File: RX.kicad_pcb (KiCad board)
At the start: 2 copper layers, 131.3 x 71.3 mm, 27 parts, among them J1 Conn_01x03, J2 Screw_Terminal_01x06, J3 Conn_01x03, J4 Conn_01x04, J5 Conn_01x04, J6 Conn_01x04, Q1 BC547, Q2 BC547, U1 ESP32-DEVKIT-V1

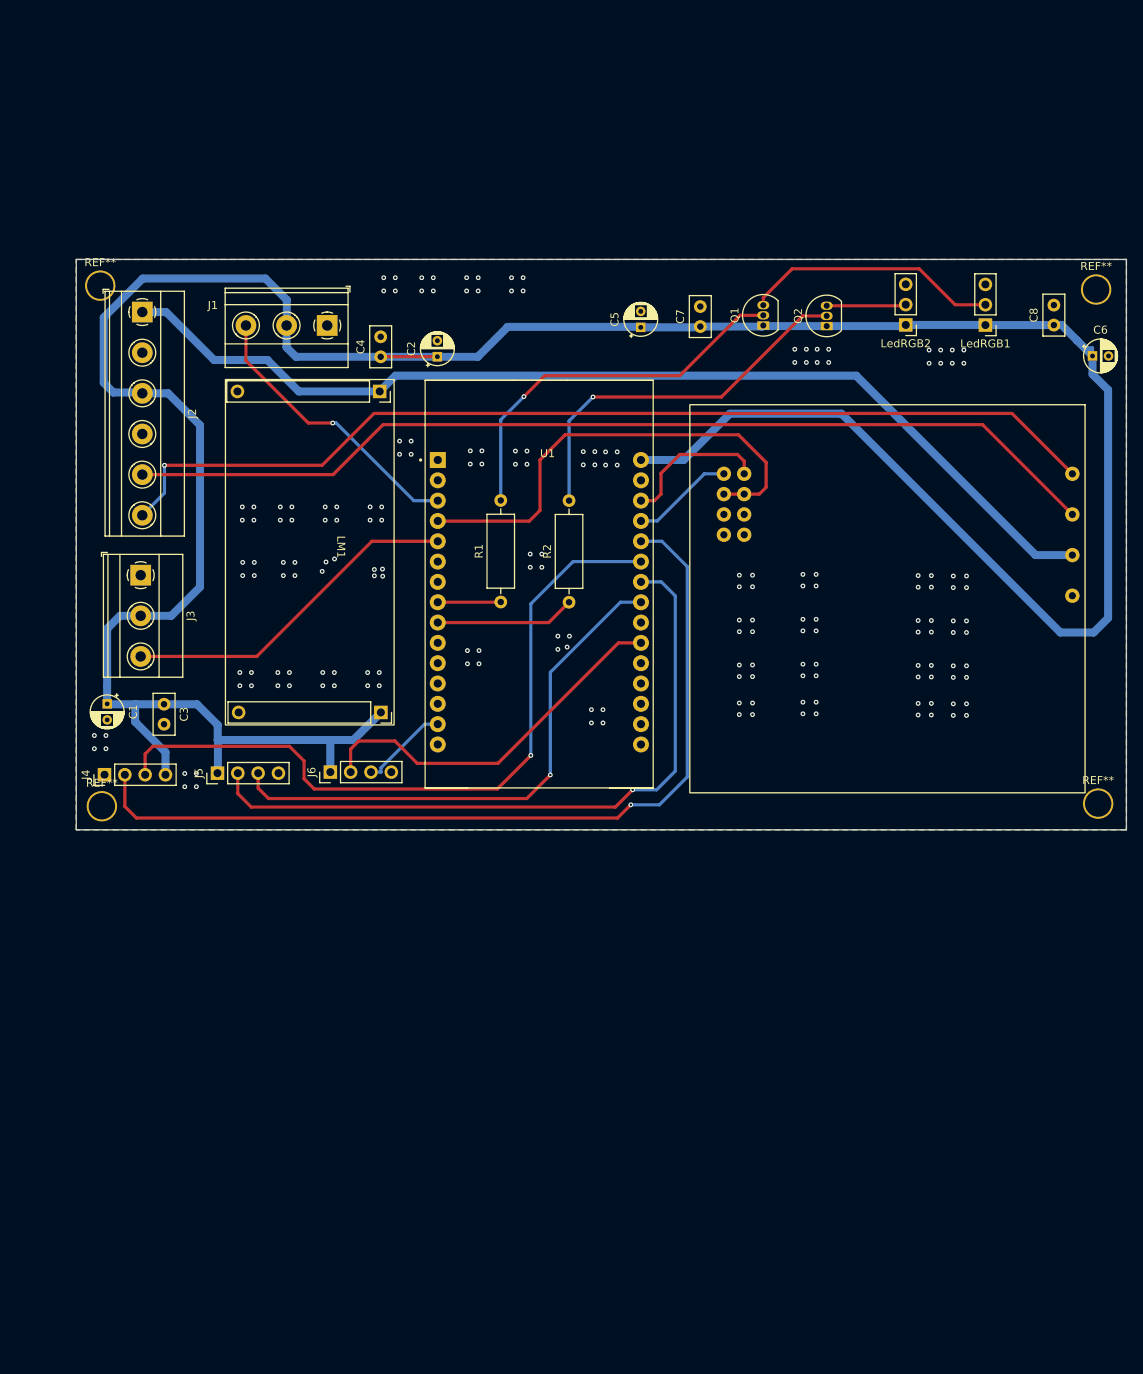
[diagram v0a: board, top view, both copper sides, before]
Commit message: Add files via upload
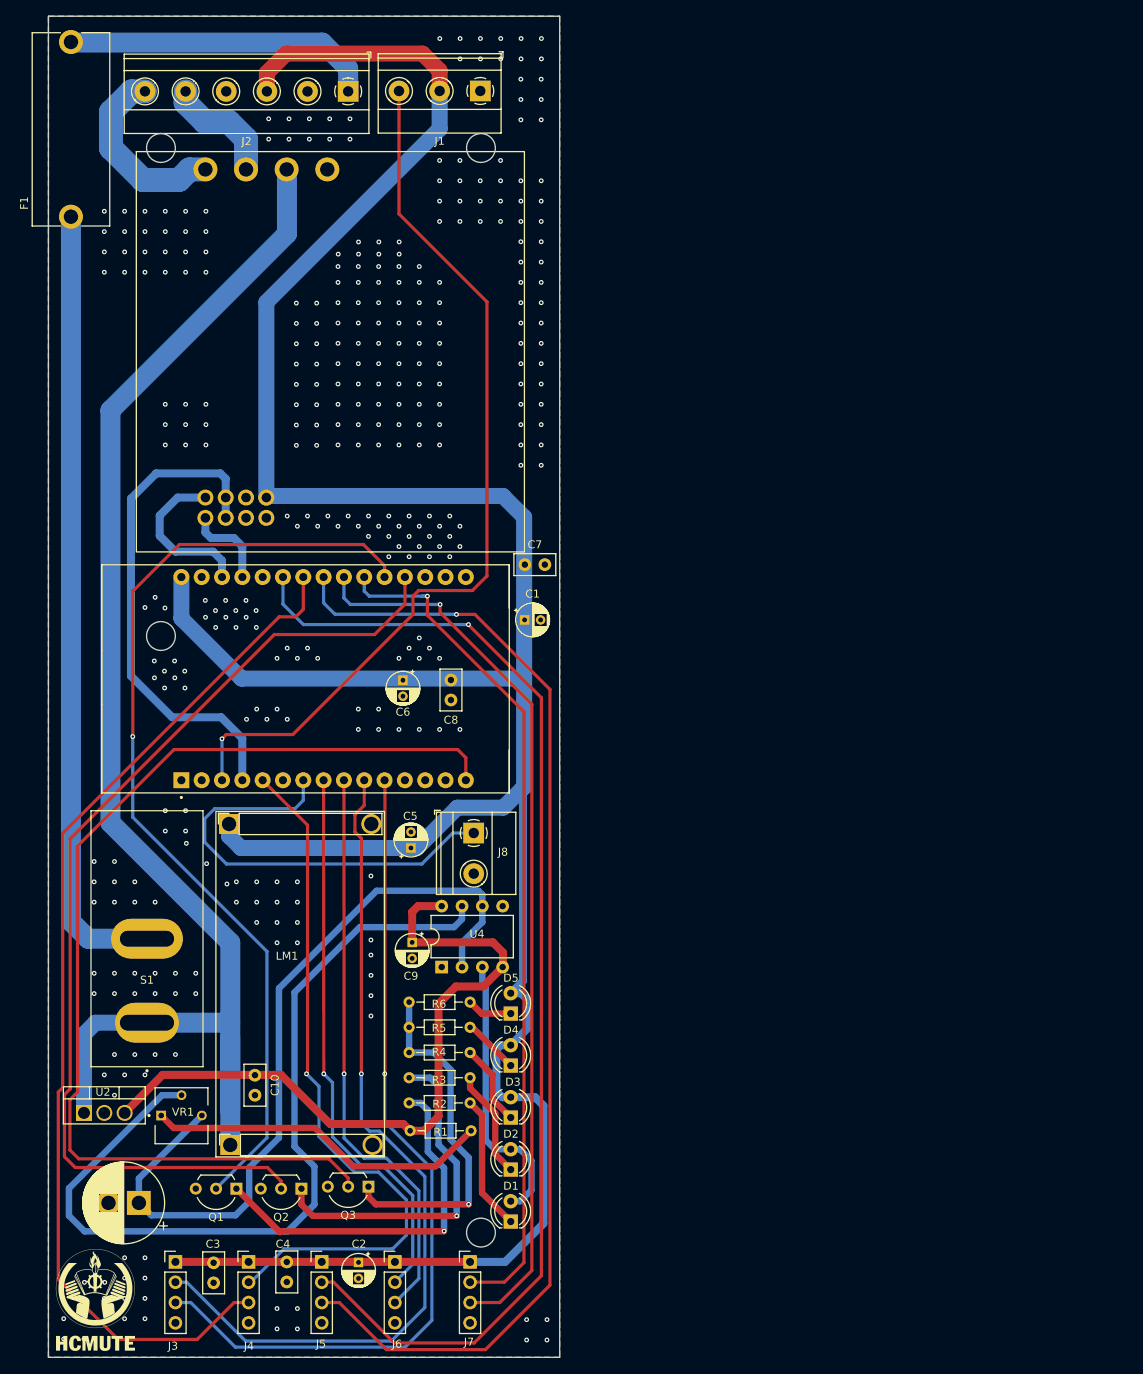
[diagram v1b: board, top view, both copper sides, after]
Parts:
- removed LedRGB1, LedRGB2: Conn_01x03, Connector_PinHeader_2.54mm:PinHeader_1x03_P2.54mm_Vertical
- removed REF** (x4): MountingHole_2.2mm_M2_DIN965_Pad, MountingHole:MountingHole_2.2mm_M2_DIN965_Pad
- added C10: C, Capacitor_THT:C_Disc_D5.0mm_W2.5mm_P2.50mm, F.Cu at (109.0, 149.9)
- added C11: 220uF, Capacitor_THT:CP_Radial_D10.0mm_P3.80mm, F.Cu at (94.5, 165.9)
- added C9: C_Polarized, Capacitor_THT:CP_Radial_D4.0mm_P2.00mm, F.Cu at (128.7, 133.3)
- added D1: LED, LED_THT:LED_D4.0mm, F.Cu at (141.0, 168.2)
- added D2: LED, LED_THT:LED_D4.0mm, F.Cu at (141.0, 161.7)
- added D3: LED, LED_THT:LED_D4.0mm, F.Cu at (141.0, 155.2)
- added D4: LED, LED_THT:LED_D4.0mm, F.Cu at (141.0, 148.7)
- added D5: LED, LED_THT:LED_D4.0mm, F.Cu at (141.0, 142.2)
- added F1: 4527, Fusebox:FUSE_4527, F.Cu at (86.0, 31.7)
- added G***: LOGO, LOGO:HCMUTE, F.Cu at (89.0, 178.0)
- added J7: Conn_01x04, Connector_PinHeader_2.54mm:PinHeader_1x04_P2.54mm_Vertical, F.Cu at (135.9, 173.2)
- added J8: Screw_Terminal_01x02, TerminalBlock_Phoenix:TerminalBlock_Phoenix_MKDS-1,5-2-5.08_1x02_P5.08mm_Horizontal, F.Cu at (136.3, 119.6)
- added Q3: NPN, Package_TO_SOT_THT:TO-92L_Inline_Wide, F.Cu at (123.2, 163.8)
- added R3: 1k, Resistor_THT:R_Axial_DIN0204_L3.6mm_D1.6mm_P7.62mm_Horizontal, F.Cu at (135.9, 150.2)
- added R4: 330, Resistor_THT:R_Axial_DIN0204_L3.6mm_D1.6mm_P7.62mm_Horizontal, F.Cu at (135.9, 147.1)
- added R5: 330, Resistor_THT:R_Axial_DIN0204_L3.6mm_D1.6mm_P7.62mm_Horizontal, F.Cu at (135.9, 143.9)
- added R6: 330, Resistor_THT:R_Axial_DIN0204_L3.6mm_D1.6mm_P7.62mm_Horizontal, F.Cu at (135.9, 140.8)
- added S1: RB141C1100, power switch:SW_POWER, F.Cu at (95.5, 132.8)
- added U3: ~, Add_DRIVER:BTS, F.Cu at (123.2, 57.2)
- added U4: ICM7555xP, Package_DIP:DIP-8_W7.62mm, F.Cu at (132.3, 136.4)
- added VR1: 3362P-1-253LF, POT_tamgiac:TRIM_3362P-1-253LF, F.Cu at (99.8, 154.9)
- J3: value Conn_01x03 -> Conn_01x04; footprint TerminalBlock_Phoenix:TerminalBlock_Phoenix_MKDS-1,5-3-5.08_1x03_P5.08mm_Horizontal -> Connector_PinHeader_2.54mm:PinHeader_1x04_P2.54mm_Vertical
- Q1, Q2: value BC547 -> NPN; footprint Package_TO_SOT_THT:TO-92_Inline -> Package_TO_SOT_THT:TO-92L_Inline_Wide
- R1, R2: value 330 -> 1k; footprint Resistor_THT:R_Axial_DIN0309_L9.0mm_D3.2mm_P12.70mm_Horizontal -> Resistor_THT:R_Axial_DIN0204_L3.6mm_D1.6mm_P7.62mm_Horizontal
- U2: value ~ -> LM7812_TO220; footprint Add_DRIVER:BTS -> Package_TO_SOT_THT:TO-220-3_Vertical
- moved Q1 126.4 mm to (106.7, 164.1), turned to 180 degrees
- moved Q2 126.2 mm to (114.8, 164.1), turned to 180 degrees
- moved U2 118.9 mm to (87.6, 154.6), turned to 0 degrees
- moved C4 113.8 mm to (113.0, 173.2), turned to -90 degrees
- moved C2 113.6 mm to (121.9, 173.3), turned to -90 degrees
- moved C6 95.3 mm to (127.5, 100.5), turned to -90 degrees
- moved C8 87.5 mm to (133.5, 100.5), turned to -90 degrees
- moved J3 86.0 mm to (99.1, 173.2), turned to 0 degrees
- moved C5 71.1 mm to (128.5, 121.5)
- moved C3 70.1 mm to (103.8, 173.4)
- moved R1 67.1 mm to (128.4, 156.8), turned to 0 degrees
- moved R2 63.8 mm to (135.9, 153.4), turned to 180 degrees
- moved J4 63.5 mm to (108.2, 173.2), turned to 0 degrees
- moved J5 62.5 mm to (117.3, 173.2), turned to 0 degrees
- moved J6 61.8 mm to (126.5, 173.2), turned to 0 degrees
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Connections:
- J2 pad 1: +12V -> VS
- J3 pad 1: GND -> +5V
- J3 pad 2: +5V -> D19
- J3 pad 3: D4 -> D21
- J4 pad 1: GND -> +5V
- J4 pad 2: D14 -> D4
- J4 pad 3: D27 -> D26
- J4 pad 4: +5V -> GND
- J5 pad 2: D26 -> D27
- J6 pad 2: D33 -> D5
- J6 pad 3: D22 -> D18
- LM1 pad 1: +12V -> +24V
- Q1 pad 1: +5V -> Net-(Q1-C)
- Q1 pad 2: Net-(Q1-B) -> D35
- Q1 pad 3: Net-(LedRGB1-Pin_2) -> GND
- Q2 pad 1: +5V -> Net-(Q2-C)
- Q2 pad 2: Net-(Q2-B) -> D34
- Q2 pad 3: Net-(LedRGB2-Pin_2) -> GND
- R1 pad 1: D5 -> +12V
- R1 pad 2: Net-(Q1-B) -> Net-(R1-Pad2)
- R2 pad 1: D18 -> Net-(D1-K)
- R2 pad 2: Net-(Q2-B) -> Net-(Q1-C)
- U1 pad 10: unconnected-(U1-D19-Pad10) -> D19
- U1 pad 11: unconnected-(U1-D21-Pad11) -> D21
- U1 pad 15: unconnected-(U1-D23-Pad15) -> D23
- U1 pad 19: unconnected-(U1-D34-Pad19) -> D34
- U1 pad 20: unconnected-(U1-D35-Pad20) -> D35
- U1 pad 21: D33 -> D32
- U1 pad 22: unconnected-(U1-D33-Pad22) -> D33
- U1 pad 7: unconnected-(U1-TX2-Pad7) -> coi
- U2 pad 1: D12 -> +24V
- U2 pad 2: D13 -> GND
- U2 pad 3: D2 -> +12V
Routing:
- net +24V: track 0.00 -> 175.2 mm
- net D23: track 0.00 -> 132.5 mm
- net D34: track 0.00 -> 126.7 mm
- net D35: track 0.00 -> 120.7 mm, vias 0 -> 1
- net D14: track 110.4 -> 0.00 mm, vias 1 -> 0
- net Net-(U4-DIS): track 0.00 -> 109.1 mm
- net M+: track 123.5 -> 14.6 mm
- net D19: track 0.00 -> 106.7 mm, vias 0 -> 1
- net D32: track 0.00 -> 106.6 mm, vias 0 -> 1
- net D21: track 0.00 -> 105.8 mm, vias 0 -> 1
- net M-: track 127.4 -> 23.8 mm, vias 1 -> 0
- net Net-(F1-Pad1): track 0.00 -> 98.5 mm
- net Net-(U4-THR): track 0.00 -> 98.3 mm
- net D15: track 35.6 -> 113.2 mm
- net D25: track 67.9 -> 144.8 mm
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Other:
- board size 131.3 x 71.3 mm -> 63.9 x 167.6 mm
